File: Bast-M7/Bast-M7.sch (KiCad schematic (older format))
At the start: 86 parts, among them J1 Conn_Battery, J2 SWD, J3 Conn_Left, J4 Conn_Right, P1 USB_C_Plug_USB2.0, Q1 TP0610L, SW1 ENABLE, SW2 ONOFF, SW3 SW_DIP_x04, SW4 RESET, U1 W25Q128JVS, U2 MIMXRT1011DAE5A, U3 MCP73831-3-OT, U4 AP63203WU-7, Y1 24Mhz, Y2 32.768KHZ

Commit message: nvcc and some capacitors fixed
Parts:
- added C? (x2): 100nF, symbol Device:C_Small
- added D?: RB521S30, symbol Device:D_Schottky
- C25, C27: value 0.22uF -> 4.7uF
- C31, C33: value 0.22uF -> 100nF
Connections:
- net +3V3: now also C5.1, C7.1, U2.39 (VDD_HIGH_IN), C?.1, C?.1, D?.2 (A); no longer R2.2, U2.31 (VDD_USB_CAP)
- net GND: now also C20.2, C25.2, C27.2, C29.2, C31.2, C33.2, C5.2, C7.2, C?.2, C?.2; no longer C20.1, C5.1, C7.1
- net VDD_SNVS_IN: now reaches U2.25 (VDD_SNVS_IN)
- net VDD_SNVS_IN: now also C20.1, D?.1 (K); no longer C20.2
- net at U2.26 (VDD_SNVS_CAP): no longer C1.1
- net at C13.1, C16.1: no longer U2.35 (VDD_HIGH_CAP)
- net at C15.1, C19.1: no longer U2.40 (NVCC_PLL)
- new net: C23.1, R2.1
- now unconnected: L1.2, U2.15 (DCDC_PSWITCH), U2.19 (DCDC_LP)
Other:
- moved on the sheet: C10, C14, C17, C18, C2, C20, C21, C22, C23, C25, C27, C29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

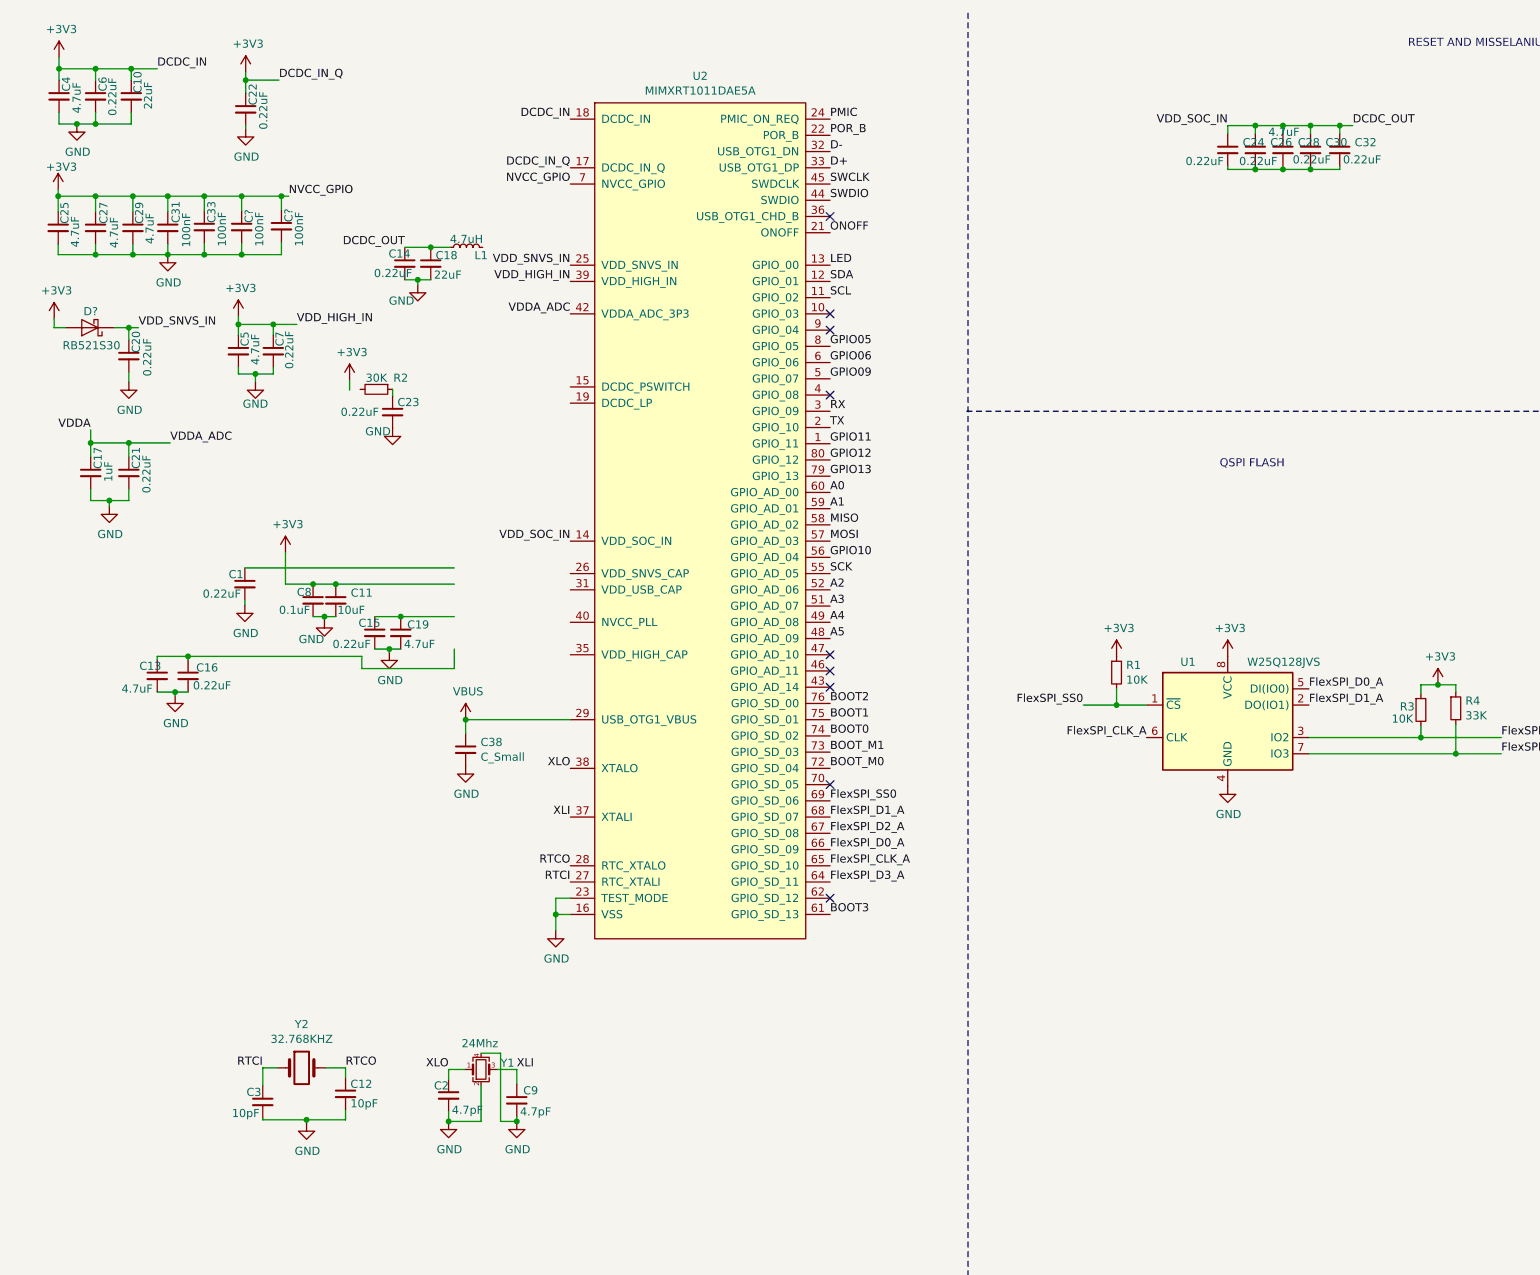
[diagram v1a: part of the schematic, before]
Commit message: fixed some pin configurations and capacitors
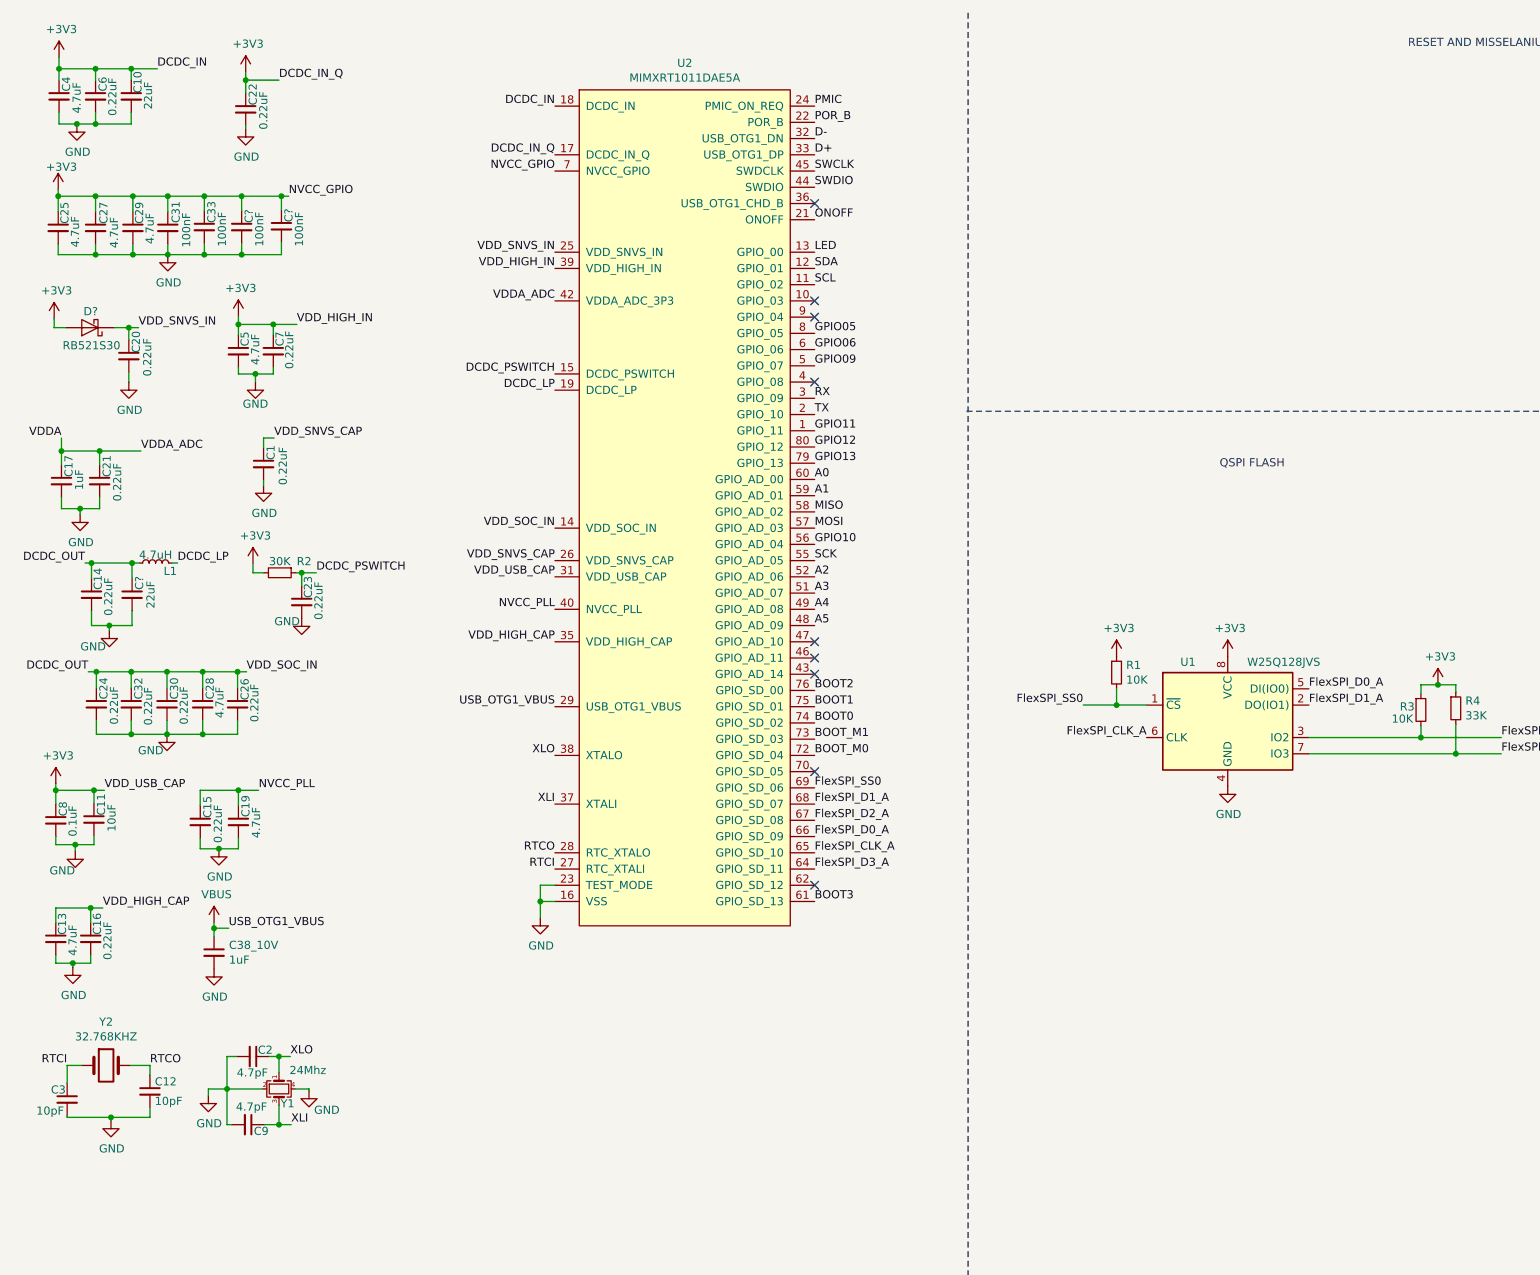
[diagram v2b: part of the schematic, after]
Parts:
- removed C18: 22uF, symbol Device:C_Small
- added C?: 22uF, symbol Device:C_Small
- C38_10V: renamed from C38; value C_Small -> 1uF
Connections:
- net +3V3: now also R2.2, U2.31 (VDD_USB_CAP)
- net DCDC_OUT: now also C?.1
- net GND: now also C24.2, C26.2, C28.2, C30.2, C32.2, C?.2
- net DCDC_PSWITCH: now reaches U2.15 (DCDC_PSWITCH)
- net DCDC_PSWITCH: now also C23.1, R2.1
- net DCDC_LP: now reaches U2.19 (DCDC_LP)
- net DCDC_LP: now also L1.2
- net VDD_SNVS_CAP: now reaches U2.26 (VDD_SNVS_CAP)
- net VDD_SNVS_CAP: now also C1.1
- net VDD_HIGH_CAP: now reaches U2.35 (VDD_HIGH_CAP)
- net VDD_HIGH_CAP: now also C13.1, C16.1
- net NVCC_PLL: now reaches U2.40 (NVCC_PLL)
- net NVCC_PLL: now also C15.1, C19.1
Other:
- moved on the sheet: C1, C11, C12, C13, C14, C15, C16, C17, C19, C2, C21, C23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

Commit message: reset and other changes
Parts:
- removed C40: 1uF, symbol Device:C
- removed SW4: RESET, symbol Switch:SW_Push
- added J?: TEST RESET, symbol Connector_Generic:Conn_02x04_Counter_Clockwise
- SW1: value ENABLE -> RESET
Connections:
- net +3V3: now also J?.4 (Pin_4)
- net GND: now also P1.S1 (SHIELD), J?.5 (Pin_5)
- net EN renamed Both
- net Both: now also J?.6 (Pin_6), J?.7 (Pin_7), J?.8 (Pin_8); no longer C41.1, SW1.2
- new net rst: C41.1, J?.1 (Pin_1), J?.2 (Pin_2), J?.3 (Pin_3), SW1.2
- no-connect marks 11 -> 10
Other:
- note added: "BOOT\n"
- note added: "CAPACITORS\n"
- note added: "MICROCONTROLLER\n"
- note added: "OSCILLATORS"
- note added: "RESET AND MISCELLANEOUS"
- note added: "SWD CONNECTOR"
- note added: "USB C"
- note added: "VREF JUMPER\n"
- note removed: "RESET AND MISSELANIUS"
- moved on the sheet: C1, C10, C11, C12, C13, C14, C15, C16, C17, C19, C2, C20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
